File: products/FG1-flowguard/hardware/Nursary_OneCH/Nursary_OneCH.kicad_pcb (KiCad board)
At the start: 2 copper layers, 29.8 x 94.8 mm, 38 parts, among them J1 FLOW1_CONN, J2 Relay1_CONN, J3 PWR_CONN, J4 FLOW2_CONN, K1 Cube_Relay, U1 ULN2003, U3 DS1307Z+, U4 DS3231M, U5 ESP32 30 Pin CP2102 Developme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, Y1 Crystal

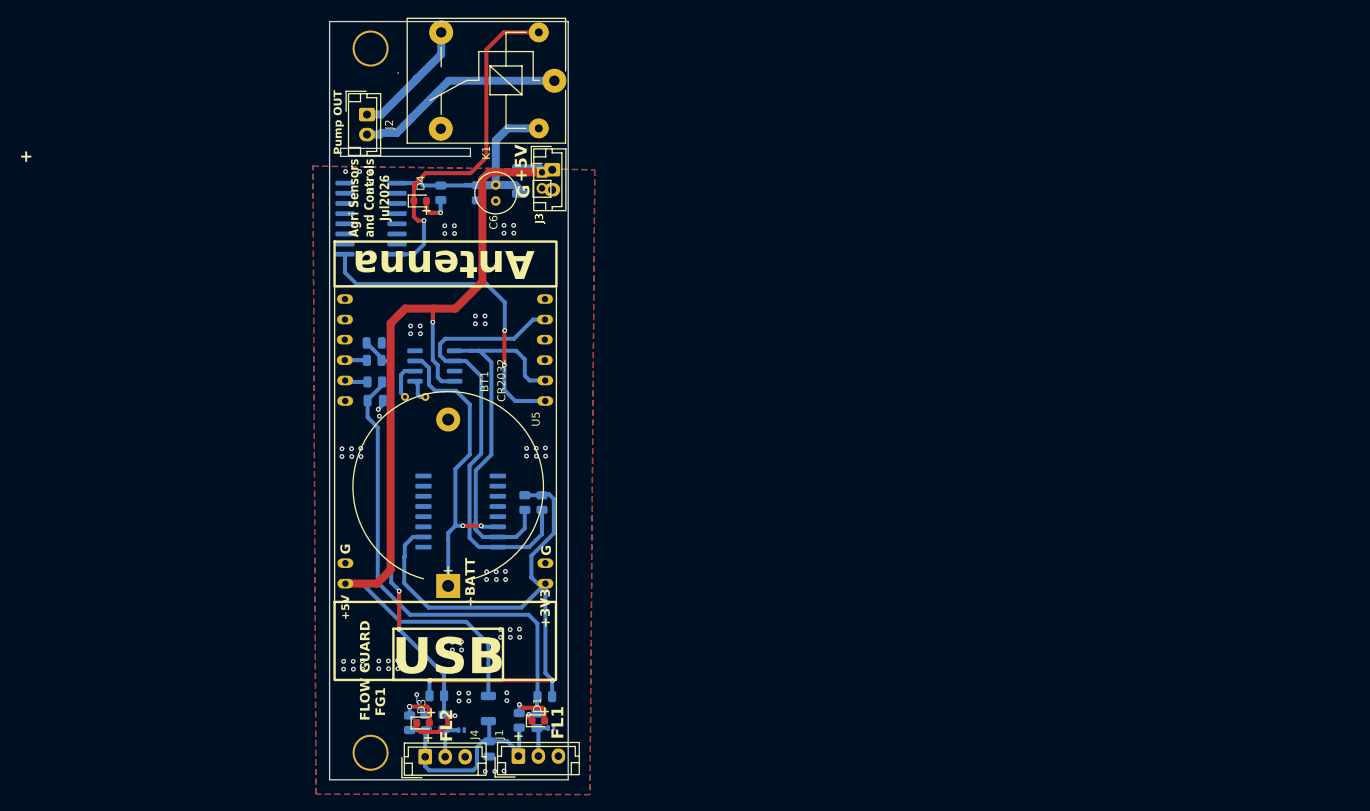
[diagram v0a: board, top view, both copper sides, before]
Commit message: Update Nursary_OneCH hardware
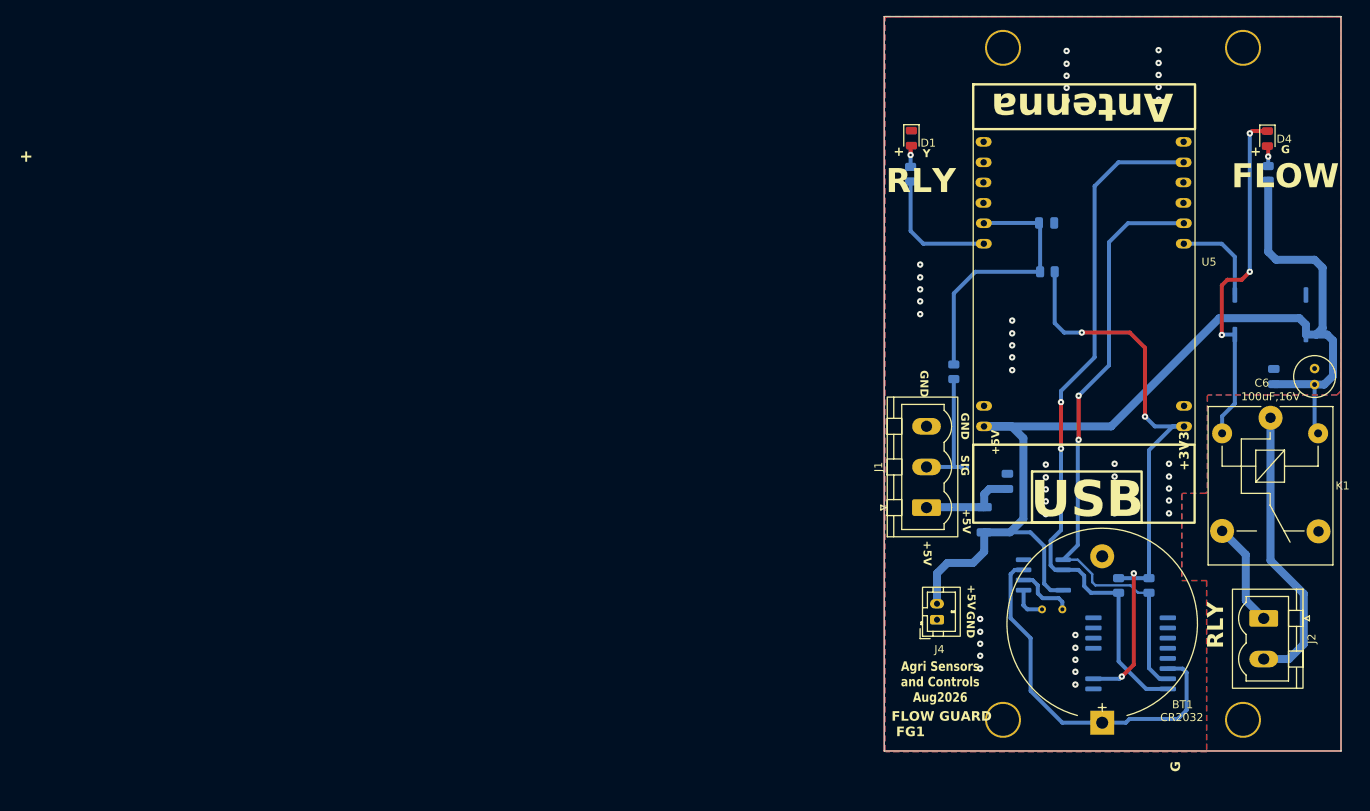
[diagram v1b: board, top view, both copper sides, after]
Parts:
- removed ., H1: MountingHole, MountingHole:MountingHole_3.2mm_M3
- removed C3: 200pF, Capacitor_SMD:C_0805_2012Metric
- removed C5: 100nF, Capacitor_SMD:C_0805_2012Metric
- removed D2, D5: PESD3V3U1UL, Diode_SMD:D_SOD-882
- removed D3: LED_GREEN_FLOW, LED_SMD:LED_0603_1608Metric
- removed F2: Polyfuse_Small, Inductor_SMD:L_1206_3216Metric
- removed J3: PWR_CONN, Connector_PinHeader_2.00mm:PinHeader_1x02_P2.00mm_Vertical
- removed J3: PWR_CONN, Connector_JST:JST_EH_B2B-EH-A_1x02_P2.50mm_Vertical
- removed R2, R6: 100E, Resistor_SMD:R_0805_2012Metric
- removed R7: 10K, Resistor_SMD:R_0805_2012Metric
- removed R8: 470E, Resistor_SMD:R_0805_2012Metric
- removed R9: 2K2, Resistor_SMD:R_0805_2012Metric
- added ?: , , F.Cu at (220.8, 47.7)
- added ?: , , F.Cu at (220.8, 131.7)
- added ?: , , F.Cu at (190.8, 131.7)
- added ?: , , F.Cu at (190.8, 47.7)
- added D6: PESD3V3U1UL, Diode_SMD:D_SOD-882, B.Cu at (185.9, 100.1)
- C2: value 200pF -> 100pF
- D1, D4: footprint LED_SMD:LED_0603_1608Metric -> LED_SMD:LED_0805_2012Metric
- J1: value FLOW1_CONN -> Conn_IN; footprint Connector_JST:JST_EH_B3B-EH-A_1x03_P2.50mm_Vertical -> Connector_Phoenix_MSTB:PhoenixContact_MSTBVA_2,5_3-G-5,08_1x03_P5.08mm_Vertical
- J2: footprint Connector_JST:JST_EH_B2B-EH-A_1x02_P2.50mm_Vertical -> Connector_Phoenix_MSTB:PhoenixContact_MSTBVA_2,5_2-G-5,08_1x02_P5.08mm_Vertical
- J4: value FLOW2_CONN -> Conn_01x02_Pin; footprint Connector_JST:JST_EH_B3B-EH-A_1x03_P2.50mm_Vertical -> Connector_JST:JST_PH_B2B-PH-K_1x02_P2.00mm_Vertical
- R1: value 2K2 -> 470E
- U1: footprint Package_SO:SOIC-16W_5.3x10.2mm_P1.27mm -> Package_SO:SOIC-16_3.9x9.9mm_P1.27mm
- moved J2 128.6 mm to (223.3, 119.0)
- moved U1 113.1 mm to (224.2, 81.0), turned to -90 degrees
- moved D4 106.2 mm to (223.8, 59.0), turned to -90 degrees
- moved C6 105.3 mm to (229.7, 89.8), turned to 90 degrees
- moved R5 103.5 mm to (223.9, 63.4), turned to 90 degrees
- moved C4 102.1 mm to (224.6, 88.8), turned to 90 degrees
- moved K1 98.9 mm to (224.2, 93.9), turned to -90 degrees
- moved C2 86.8 mm to (196.2, 69.6)
- moved D1 86.5 mm to (179.3, 59.0), turned to -90 degrees
- moved U4 85.6 mm to (206.7, 123.4)
- moved R3 84.0 mm to (179.2, 63.5)
- moved Y1 83.9 mm to (198.2, 117.9)
- moved BT1 83.5 mm to (203.2, 132.0)
- moved R4 82.3 mm to (196.3, 75.7)
- moved U5 82.2 mm to (213.4, 95.0)
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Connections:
- net /FLOW1_CONN renamed /FLOW1_CON
- C2 pad 1: /FLOW1_PROT -> /FLOW1_MCU
- C4 pad 1: +5VR -> +5V
- C6 pad 1: +5VR -> +5V
- D1 pad 1: /FLOW1_PROT -> GND
- J4 pad 1: +5VP -> GND
- J4 pad 2: /FLOW2_CONN -> +5V
- K1 pad 5: +5VR -> +5V
- R1 pad 1: /FLOW1_PROT -> /FLOW1_MCU
- R3 pad 1: +5VP -> /FLOW1_LED_MCU
- R4 pad 2: /FLOW1_PROT -> /FLOW1_MCU
- R5 pad 1: +5VR -> +5V
- U1 pad 9: +5VR -> +5V
- U5 pad 19: /FLOW2_MCU -> unconnected-(U5-D34/Input_only-Pad19)
- U5 pad 21: unconnected-(U5-D32-Pad21) -> /FLOW1_LED_MCU
- Y1 pad 1: Net-(U3-X1) -> Net-(U3-X2)
- Y1 pad 2: Net-(U3-X2) -> Net-(U3-X1)
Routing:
- net /FLOW1_PROT: track 61.7 -> 0.00 mm, vias 1 -> 0
- net /FLOW2_PROT: track 59.4 -> 0.00 mm, vias 3 -> 0
- net /SCL: track 56.0 -> 88.9 mm, vias 0 -> 2
- net /FLOW1_MCU: track 2.74 -> 33.9 mm
- net /SDA: track 47.5 -> 77.7 mm, vias 0 -> 2
- net /RELAY1_MCU: track 40.5 -> 11.8 mm, vias 2 -> 0
- net +5VR: track 28.5 -> 0.00 mm
- net +5V: track 115.8 -> 141.7 mm, vias 1 -> 0
- net +5VP: track 28.7 -> 12.0 mm
- net /FLOW1_LED_MCU: track 0.00 -> 16.0 mm
- net /FLOW1_CON: track 4.99 -> 15.4 mm
- net Net-(J2-Pin_2): track 26.2 -> 35.8 mm
- net /BATT: track 39.5 -> 46.5 mm, vias 2 -> 0
- net GND: track 5.72 -> 0.00 mm, vias 75 -> 45
- net Net-(D3-A): track 5.46 -> 0.00 mm, vias 3 -> 0
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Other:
- board size 29.8 x 94.8 mm -> 57.1 x 91.8 mm
- board text added: "Agri Sensors and Controls Aug2026"
- board text added: "FLOW"
- board text added: "GND"
- board text added: "RLY"
- board text added: "SIG"
- board text added: "Y"
- board text removed: "+BATT"
- board text removed: "Agri Sensors and Controls Jul2026"
- board text removed: "FL1"
- board text removed: "FL2"
- board text removed: "Pump OUT"
